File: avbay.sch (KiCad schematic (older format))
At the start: 2 parts, among them U1 STM32F411RE_LQFP64, U2 XBEE

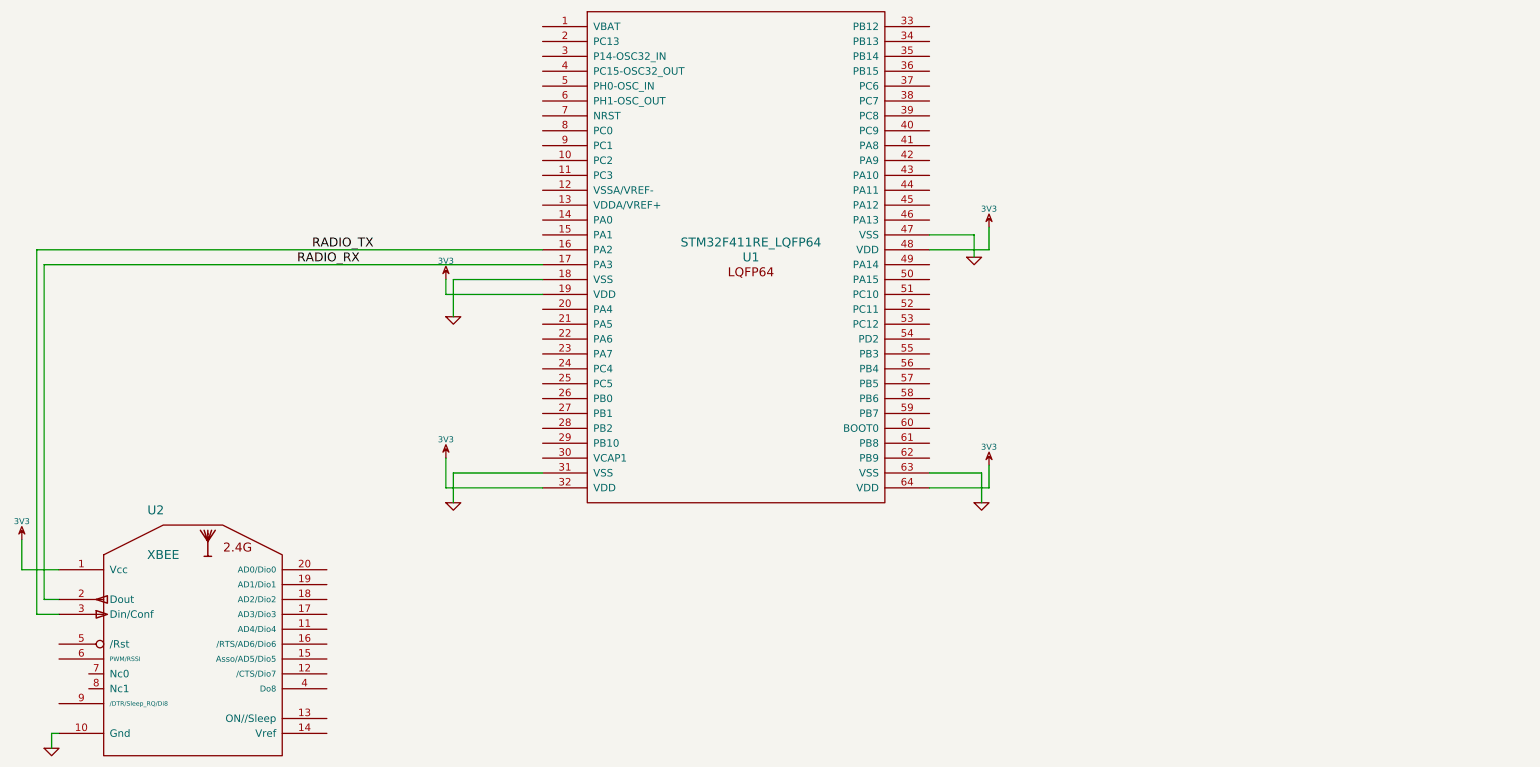
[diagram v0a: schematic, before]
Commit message: Prototype made
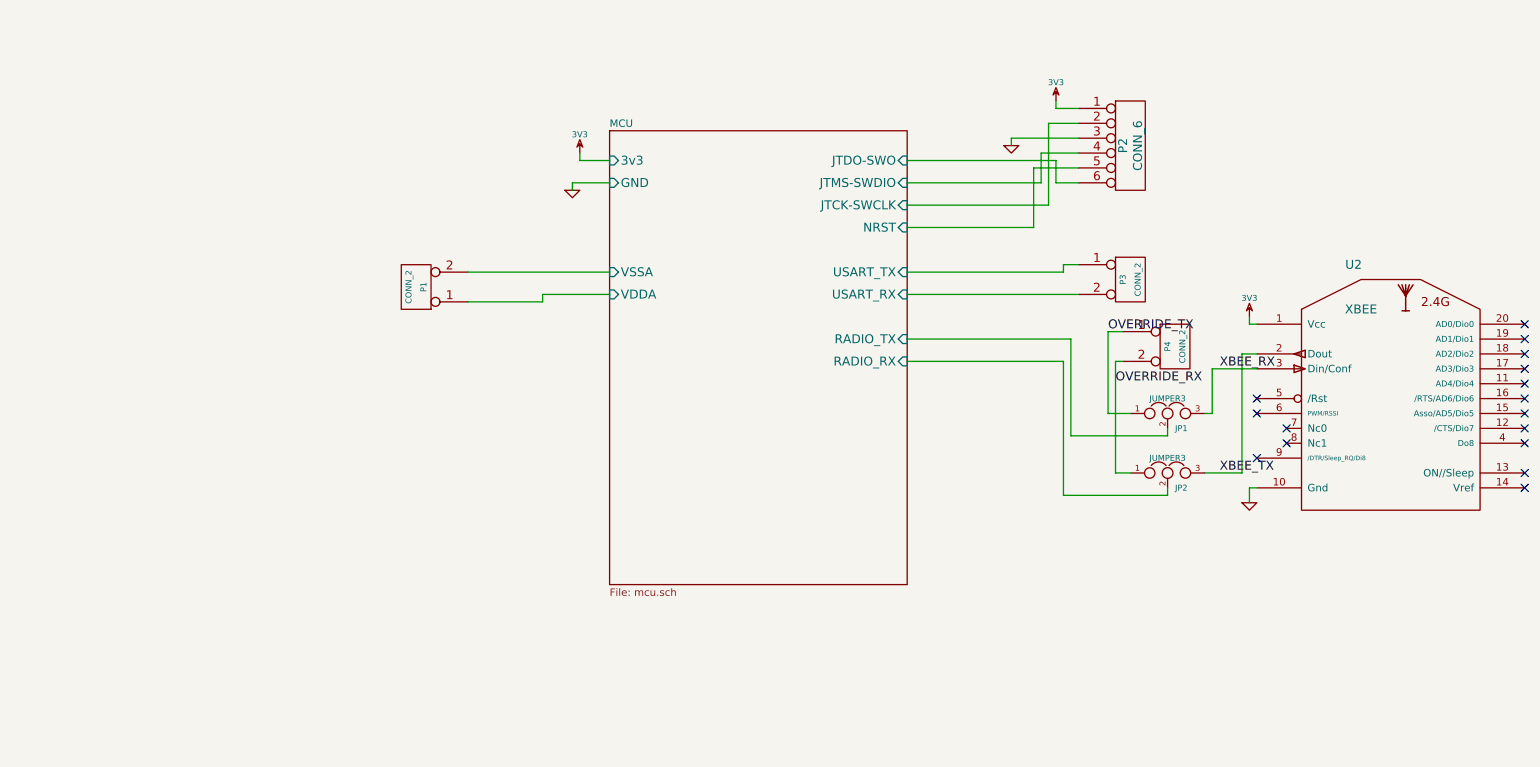
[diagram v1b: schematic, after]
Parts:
- removed U1: STM32F411RE_LQFP64, symbol STM32F411RE_LQFP64
- added JP1, JP2: JUMPER3, ~, symbol JUMPER3
- added P1, P3, P4: CONN_2, symbol CONN_2
- added P2: CONN_6, symbol CONN_6
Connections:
- net 3V3: now also P2.1
- net GND: now also P2.3
- net RADIO_RX renamed XBEE_TX
- net XBEE_TX: now also JP2.3
- net RADIO_TX renamed XBEE_RX
- net XBEE_RX: now also JP1.3
- new net MCU/JTCK-SWCLK: P2.2
- new net MCU/JTDO-SWO: P2.6
- new net MCU/JTMS-SWDIO: P2.4
- new net MCU/NRST: P2.5
- new net MCU/RADIO_RX: JP2.2
- new net MCU/RADIO_TX: JP1.2
- new net MCU/USART_RX: P3.2 (PM)
- new net MCU/USART_TX: P3.1 (P1)
- new net MCU/VDDA: P1.1 (P1)
- new net MCU/VSSA: P1.2 (PM)
- new net OVERRIDE_RX: JP2.1, P4.2 (PM)
- new net OVERRIDE_TX: JP1.1, P4.1 (P1)
- no-connect marks 0 -> 16
